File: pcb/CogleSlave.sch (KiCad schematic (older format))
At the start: 7 parts, among them P1 CONN_01X04, P2 CONN_01X04, P3 CONN_01X08, U1 PCF8591T

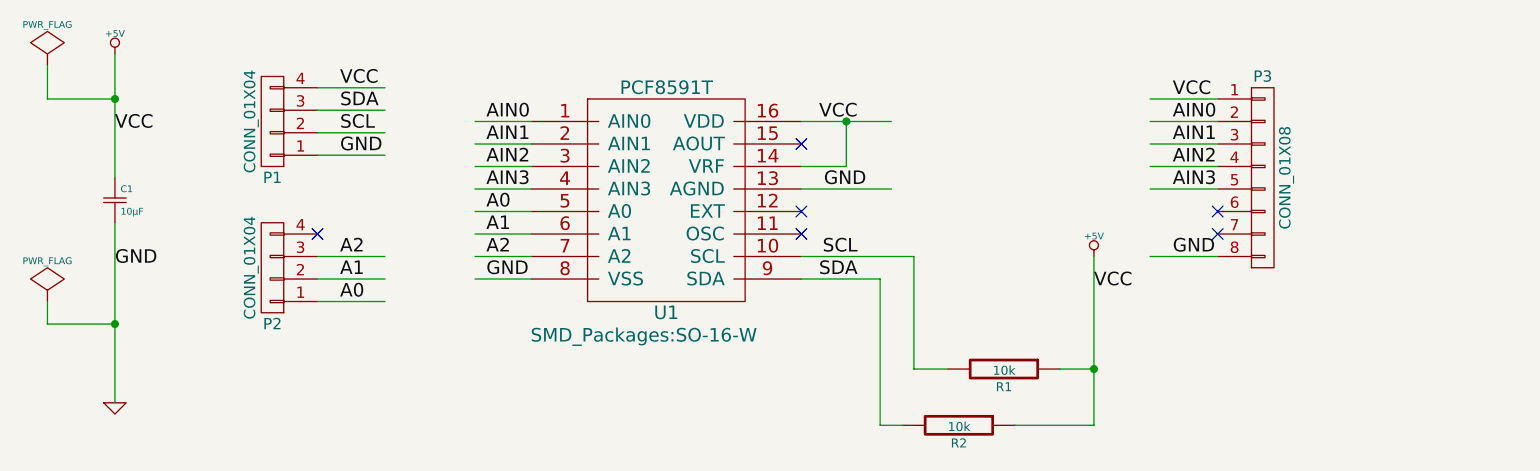
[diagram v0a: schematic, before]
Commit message: 基板レイアウトを修正 1.2
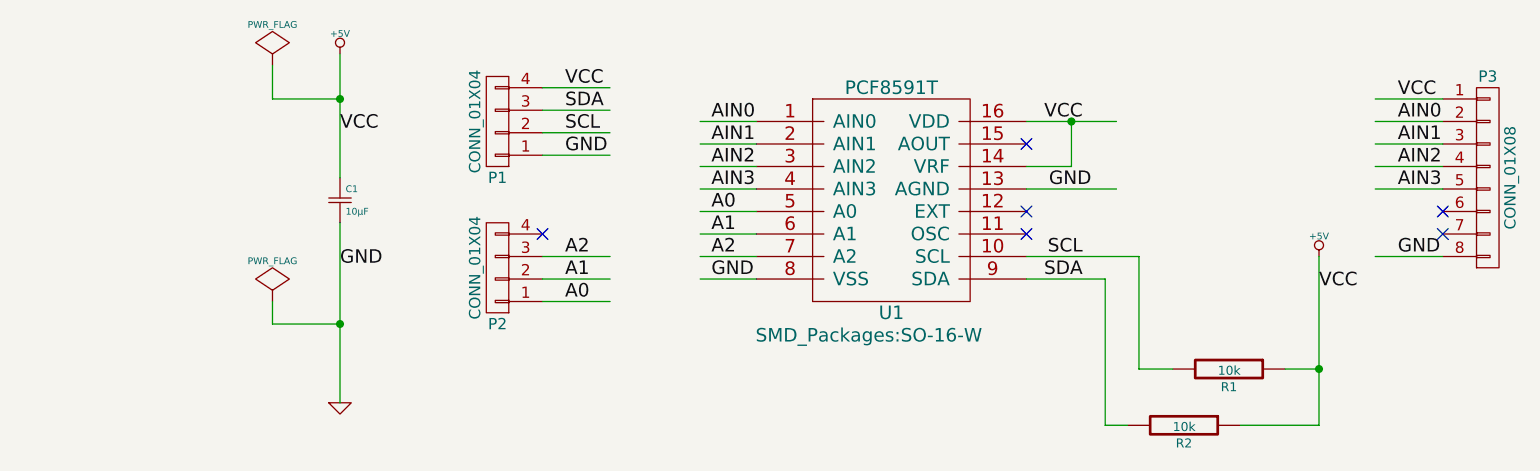
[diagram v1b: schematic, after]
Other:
- moved on the sheet: C1, P1, P2, P3, R1, R2, U1
